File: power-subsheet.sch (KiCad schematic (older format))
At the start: 42 parts, among them CON1 BARREL_JACK, SW3 ON/OFF, T1 PMV45EN2, T2 PMV45EN2, T3 PMV45EN2, T4 PMV45EN2, U11 LT1085, U12 NCP1117ST50T3G_MountingTab, U13 MAX1721, U14 NCP1117ST50T3G_MountingTab, U15 MAX6820, U16 NCP1117ST50T3G_MountingTab, U17 MAX6820, U18 LT3580

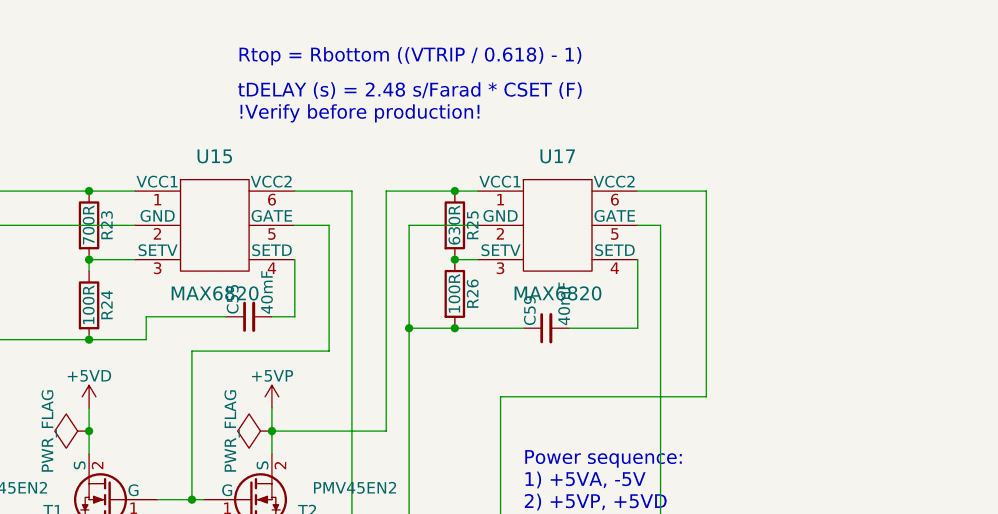
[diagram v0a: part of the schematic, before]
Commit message: before initial DRC
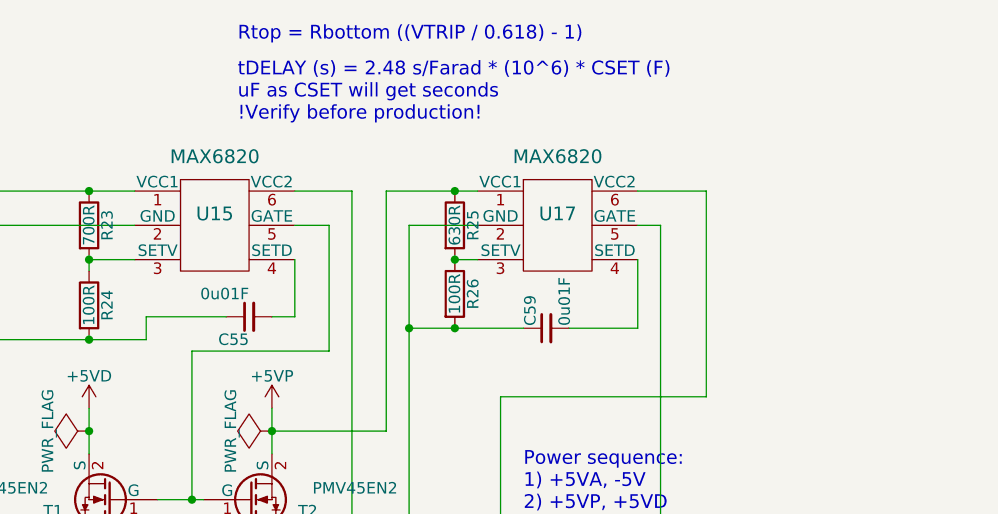
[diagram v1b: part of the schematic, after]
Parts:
- C55, C59: value 40mF -> 0u01F
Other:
- note added: "tDELAY (s) = 2.48 s/Farad * (10^6) * CSET (F)\nuF as CSET will get seconds\n!Verify before production!"
- note removed: "tDELAY (s) = 2.48 s/Farad * CSET (F)\n!Verify before production!"
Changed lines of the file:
@@
 $EndDescr
 $Comp
-L +12VA #PWR092
+L +12VA #PWR093
 U 1 1 580C6FB9
 P 7100 3150
-F 0 "#PWR092" H 7100 3000 50  0001 C CNN
+F 0 "#PWR093" H 7100 3000 50  0001 C CNN
 F 1 "+12VA" H 7100 3290 50  0000 C CNN
 F 2 "" H 7100 3150 50  0000 C CNN
@@
 $EndComp
 $Comp
-L -12VA #PWR093
+L -12VA #PWR094
 U 1 1 580C6FCD
 P 7950 3150
-F 0 "#PWR093" H 7950 3000 50  0001 C CNN
+F 0 "#PWR094" H 7950 3000 50  0001 C CNN
 F 1 "-12VA" H 7950 3290 50  0000 C CNN
 F 2 "" H 7950 3150 50  0000 C CNN
@@
 $EndComp
 $Comp
-L +5VD #PWR094
+L +5VD #PWR095
 U 1 1 580C6FE1
 P 5100 2250
-F 0 "#PWR094" H 5100 2100 50  0001 C CNN
+F 0 "#PWR095" H 5100 2100 50  0001 C CNN
 F 1 "+5VD" H 5100 2390 50  0000 C CNN
 F 2 "" H 5100 2250 50  0000 C CNN
@@
 $EndComp
 $Comp
-L +5VA #PWR095
+L +5VA #PWR096
 U 1 1 580C6FF5
 P 3900 2650
-F 0 "#PWR095" H 3900 2500 50  0001 C CNN
+F 0 "#PWR096" H 3900 2500 50  0001 C CNN
 F 1 "+5VA" H 3900 2790 50  0000 C CNN
 F 2 "" H 3900 2650 50  0000 C CNN
@@
 $EndComp
 $Comp
-L GNDREF #PWR096
+L GNDREF #PWR097
 U 1 1 580C7009
 P 2300 4000
-F 0 "#PWR096" H 2300 3750 50  0001 C CNN
+F 0 "#PWR097" H 2300 3750 50  0001 C CNN
 F 1 "GNDREF" H 2300 3850 50  0000 C CNN
 F 2 "" H 2300 4000 50  0000 C CNN
@@
 $EndComp
 $Comp
-L +5VP #PWR097
+L +5VP #PWR098
 U 1 1 580B2C17
 P 5900 2250
-F 0 "#PWR097" H 5900 2100 50  0001 C CNN
+F 0 "#PWR098" H 5900 2100 50  0001 C CNN
 F 1 "+5VP" H 5900 2390 50  0000 C CNN
 F 2 "" H 5900 2250 50  0000 C CNN
@@
 $EndComp
 $Comp
-L -5V #PWR3
+L -5V #PWR103
 U 1 1 580B2D1F
 P 4050 1750
-F 0 "#PWR3" H 4050 1850 50  0001 C CNN
+F 0 "#PWR103" H 4050 1850 50  0001 C CNN
 F 1 "-5V" H 4050 1900 50  0000 C CNN
 F 2 "" H 4050 1750 50  0000 C CNN
@@
 U 1 1 580B3CA2
 P 7150 1450
-F 0 "U17" H 7150 1750 60  0000 C CNN
-F 1 "MAX6820" H 7150 1150 60  0000 C CNN
+F 0 "U17" H 7150 1500 60  0000 C CNN
+F 1 "MAX6820" H 7150 1750 60  0000 C CNN
 F 2 "TO_SOT_Packages_SMD:SOT-23-6_Handsoldering" H 6900 1400 60  0001 C CNN
 F 3 "https://datasheets.maximintegrated.com/en/ds/MAX6819-MAX6820.pdf" H 7250 850 60  0001 C CNN
@@
 U 1 1 580B3D03
 P 5650 1450
-F 0 "U15" H 5650 1750 60  0000 C CNN
-F 1 "MAX6820" H 5650 1150 60  0000 C CNN
+F 0 "U15" H 5650 1500 60  0000 C CNN
+F 1 "MAX6820" H 5650 1750 60  0000 C CNN
 F 2 "TO_SOT_Packages_SMD:SOT-23-6_Handsoldering" H 5400 1400 60  0001 C CNN
 F 3 "https://datasheets.maximintegrated.com/en/ds/MAX6819-MAX6820.pdf" H 5750 850 60  0001 C CNN
@@
 $EndComp
 $Comp
-L GNDREF #PWR098
+L GNDREF #PWR099
 U 1 1 580B63E1
 P 7100 4850
-F 0 "#PWR098" H 7100 4600 50  0001 C CNN
+F 0 "#PWR099" H 7100 4600 50  0001 C CNN
 F 1 "GNDREF" H 7100 4700 50  0000 C CNN
 F 2 "" H 7100 4850 50  0000 C CNN
@@
 U 1 1 580B9EE1
 P 5800 1850
-F 0 "C55" H 5810 1920 50  0000 L CNN
-F 1 "40mF" H 5810 1770 50  0000 L CNN
+F 0 "C55" V 5700 1850 50  0000 L CNN
+F 1 "0u01F" V 5900 1850 50  0000 L CNN
 F 2 "Capacitors_SMD:C_0603_HandSoldering" H 5800 1850 50  0001 C CNN
 F 3 "" H 5800 1850 50  0000 C CNN
@@
 $EndComp
 Text Notes 5750 1000 0    60   ~ 0
-tDELAY (s) = 2.48 s/Farad * CSET (F)\n!Verify before production!
-Text Notes 5750 750  0    60   ~ 0
+tDELAY (s) = 2.48 s/Farad * (10^6) * CSET (F)\nuF as CSET will get seconds\n!Verify before production!
+Text Notes 5750 650  0    60   ~ 0
 Rtop = Rbottom ((VTRIP / 0.618) - 1) \n
 Wire Wire Line
@@
 P 7100 1900
 F 0 "C59" H 7110 1970 50  0000 L CNN
-F 1 "40mF" H 7110 1820 50  0000 L CNN
+F 1 "0u01F" H 7110 1820 50  0000 L CNN
 F 2 "Capacitors_SMD:C_0603_HandSoldering" H 7100 1900 50  0001 C CNN
 F 3 "" H 7100 1900 50  0000 C CNN
@@
 Connection ~ 6900 3800
 $Comp
-L PWR_FLAG #FLG099
+L PWR_FLAG #FLG0100
 U 1 1 580C134B
 P 7100 3300
-F 0 "#FLG099" H 7100 3395 50  0001 C CNN
+F 0 "#FLG0100" H 7100 3395 50  0001 C CNN
 F 1 "PWR_FLAG" H 7100 3480 50  0000 C CNN
 F 2 "" H 7100 3300 50  0000 C CNN
@@
 $EndComp
 $Comp
-L PWR_FLAG #FLG0100
+L PWR_FLAG #FLG0101
 U 1 1 580C1455
 P 7950 3300
-F 0 "#FLG0100" H 7950 3395 50  0001 C CNN
+F 0 "#FLG0101" H 7950 3395 50  0001 C CNN
 F 1 "PWR_FLAG" H 7950 3480 50  0000 C CNN
 F 2 "" H 7950 3300 50  0000 C CNN
@@
 Connection ~ 4050 1800
 $Comp
-L PWR_FLAG #FLG0101
+L PWR_FLAG #FLG0102
 U 1 1 580C1C36
 P 5900 2350
-F 0 "#FLG0101" H 5900 2445 50  0001 C CNN
+F 0 "#FLG0102" H 5900 2445 50  0001 C CNN
 F 1 "PWR_FLAG" H 5900 2530 50  0000 C CNN
 F 2 "" H 5900 2350 50  0000 C CNN
@@
 $EndComp
 $Comp
-L PWR_FLAG #FLG0102
+L PWR_FLAG #FLG0103
 U 1 1 580C1CC5
 P 5100 2350
-F 0 "#FLG0102" H 5100 2445 50  0001 C CNN
+F 0 "#FLG0103" H 5100 2445 50  0001 C CNN
 F 1 "PWR_FLAG" H 5100 2530 50  0000 C CNN
 F 2 "" H 5100 2350 50  0000 C CNN
@@
 NoConn ~ 4250 2650
 $Comp
-L PWR_FLAG #FLG0103
+L PWR_FLAG #FLG0104
 U 1 1 580C30D2
 P 2450 3800
-F 0 "#FLG0103" H 2450 3895 50  0001 C CNN
+F 0 "#FLG0104" H 2450 3895 50  0001 C CNN
 F 1 "PWR_FLAG" H 2450 3980 50  0000 C CNN
 F 2 "" H 2450 3800 50  0000 C CNN
@@
 Connection ~ 2450 3800
 $Comp
-L PWR_FLAG #FLG0104
+L PWR_FLAG #FLG0105
 U 1 1 580C4729
 P 2600 4000
-F 0 "#FLG0104" H 2600 4095 50  0001 C CNN
+F 0 "#FLG0105" H 2600 4095 50  0001 C CNN
 F 1 "PWR_FLAG" H 2600 4180 50  0000 C CNN
 F 2 "" H 2600 4000 50  0000 C CNN
